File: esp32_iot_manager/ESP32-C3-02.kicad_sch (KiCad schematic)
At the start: 0 parts

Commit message: esp32 page and datasheets
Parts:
- added C10, C13, C14, C8: 0.1u, Capacitor_THT:C_Disc_D3.0mm_W2.0mm_P2.50mm, symbol PCM_SL_Devices:Capacitor_NP
- added C11: 1u, Capacitor_THT:C_Disc_D3.0mm_W2.0mm_P2.50mm, symbol PCM_SL_Devices:Capacitor_NP
- added C13, C7: 10u, symbol Device:C_Polarized
- added C9: 4.7u, symbol Device:C_Polarized
- added J3: GSD090012SEU, GSD090012SEU:AMPHENOL_GSD090012SEU, symbol GSD090012SEU:GSD090012SEU
- added LED5: LTST-C170GKT, LEDC2012X120N, symbol LTST-C170GKT:LTST-C170GKT
- added LED6: LTST-C170KRKT, LEDC2012X120N, symbol LTST-C170KRKT:LTST-C170KRKT
- added R11: 1K, Resistor_THT:R_Axial_DIN0207_L6.3mm_D2.5mm_P10.16mm_Horizontal, symbol PCM_SL_Resistors:Resistor
- added R12: 22.1K, symbol Device:R
- added R13: 47.5K, symbol Device:R
- added R15, R16, R20, R22: 50, Resistor_THT:R_Axial_DIN0207_L6.3mm_D2.5mm_P10.16mm_Horizontal, symbol PCM_SL_Resistors:Resistor
- added R15, R18: 470, symbol Device:R
- added R19: 10K, Resistor_THT:R_Axial_DIN0207_L6.3mm_D2.5mm_P10.16mm_Horizontal, symbol PCM_SL_Resistors:Resistor
- added U3: ESP32-C3-WROOM-02-H4, ESP32-C3-WROOM-02-H4:MODULE_ESP32-C3-WROOM-02-H4, symbol ESP32-C3-WROOM-02-H4:ESP32-C3-WROOM-02-H4
- added U4: CP2102N-Axx-xQFN20, Package_DFN_QFN:SiliconLabs_QFN-20-1EP_3x3mm_P0.5mm, symbol Interface_USB:CP2102N-Axx-xQFN20
- added U5: USBLC6-2P6, PCM_Package_TO_SOT_SMD_AKL:SOT-666, symbol PCM_Diode_TVS_AKL:USBLC6-2P6
- added U6: W25Q32JVSSIQ, W25Q32JVSSIQ:SOIC127P790X216-8N, symbol W25Q32JVSSIQ:W25Q32JVSSIQ
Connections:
- new net: R11.1, U4.9 (~{RST})
- new net: C11.2, R12.2, R13.1, U4.8 (VBUS)
- new net: R20.2, U3.5 (IO6)
- new net: LED6.1 (K), R18.1
- new net: LED5.1 (K), R15.2
- new net: R18.2, U4.19 (~{RXT}/GPIO.3)
- new net: R15.1, U4.20 (~{TXT}/GPIO.2)
- new net: R15.1, U3.6 (IO7)
- new net: J3.7 (DAT0), R16.2
- new net: C14.2, U6.8 (VCC)
- new net: R22.1, U6.2 (DO(IO1))
- new net 3.3V: C10.1, C13.1, C13.2, C7.1, C8.2, C9.1, J3.4 (VDD1), LED5.2 (A), LED6.2 (A), R11.2, R19.1, U3.1 (3V3), U4.6 (VDD), U4.7 (VREGIN), U6.3 (~{WP}(IO2)), U6.7 (~{HOLD}/~{RESET}(IO3))
- new net BOOT: U3.8 (IO9)
- new net CS: U3.10 (IO10), U6.1 (~{CS})
- new net CS_SD: J3.1 (CD/DAT3), R19.2, U3.18 (IO0)
- new net DTS: U4.15 (~{CTS})
- new net EN: U3.2 (EN)
- new net GND: C10.2, C11.1, C13.1, C13.2, C14.1, C7.2, C8.1, C9.2, J3.3 (VSS1), J3.6 (VSS2), J3.8 (DAT1), J3.9 (DAT2), J3.G1 (SHIELD_GND), J3.G2 (SHIELD_GND), J3.G3 (SHIELD_GND), J3.G4 (SHIELD_GND), R13.2, U3.19 (GND), U3.20 (GND), U3.21 (GND), U3.22 (GND), U3.23 (GND), U3.24 (GND), U3.25 (GND), U3.26 (GND), U3.27 (GND), U3.28 (GND), U3.29 (GND), U3.30 (GND), U3.31 (GND), U3.32 (GND), U3.33 (GND), U3.34 (GND), U3.35 (GND), U3.36 (GND), U3.37 (GND), U3.38 (GND), U3.39 (GND), U3.9 (GND), U4.12 (GND), U4.21 (GND), U4.3 (GND), U5.2 (VN), U6.4 (GND)
- new net GPI019: U3.14 (IO19)
- new net GPIO18: U3.13 (IO18)
- new net GPIO8: U3.7 (IO8)
- new net MIC_OUT: U3.4 (IO5)
- new net MISO_DO: R16.1, R22.2, U3.16 (IO2)
- new net MOSI_DI: J3.2 (CMD), R15.2, U6.5 (DI(IO0))
- new net PHOTO_C: U3.17 (IO1)
- new net RTS: U4.16 (~{RTS})
- new net RX_TX: U3.11 (RXD), U4.17 (RXD)
- new net SCL: U3.15 (IO3)
- new net SCLK: J3.5 (CLK), R20.1, U6.6 (CLK)
- new net SDA: U3.3 (IO4)
- new net TX_RX: U3.12 (TXD), U4.18 (TXD)
- new net USB_DATA+: U4.4 (D+), U5.3 (L2)
- new net USB_DATA-: U4.5 (D-), U5.1 (L1)
- new net USB_DN: U5.6 (L1)
- new net USB_DP: U5.4 (L2)
- new net V_BUS: R12.1, U5.5 (VP)
- no-connect marks 0 -> 7
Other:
- note added: "ESP32"
- note added: "Flash Memory"
- note added: "SD Card"
- note added: "USB Module"

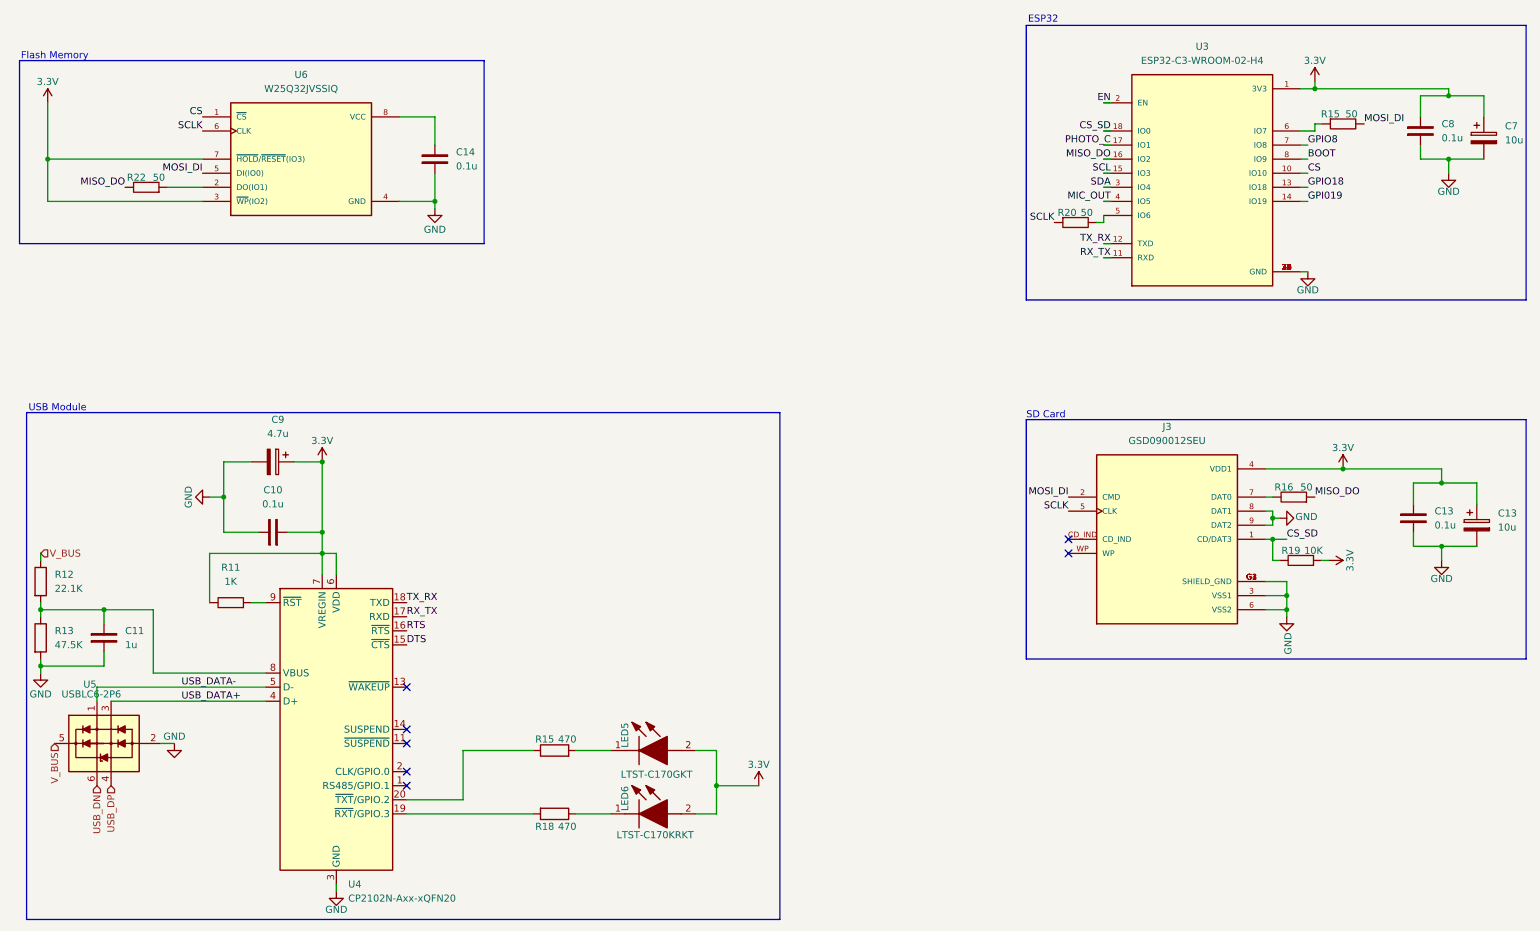
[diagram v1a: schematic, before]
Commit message: finished esp32 sheet, next sensors
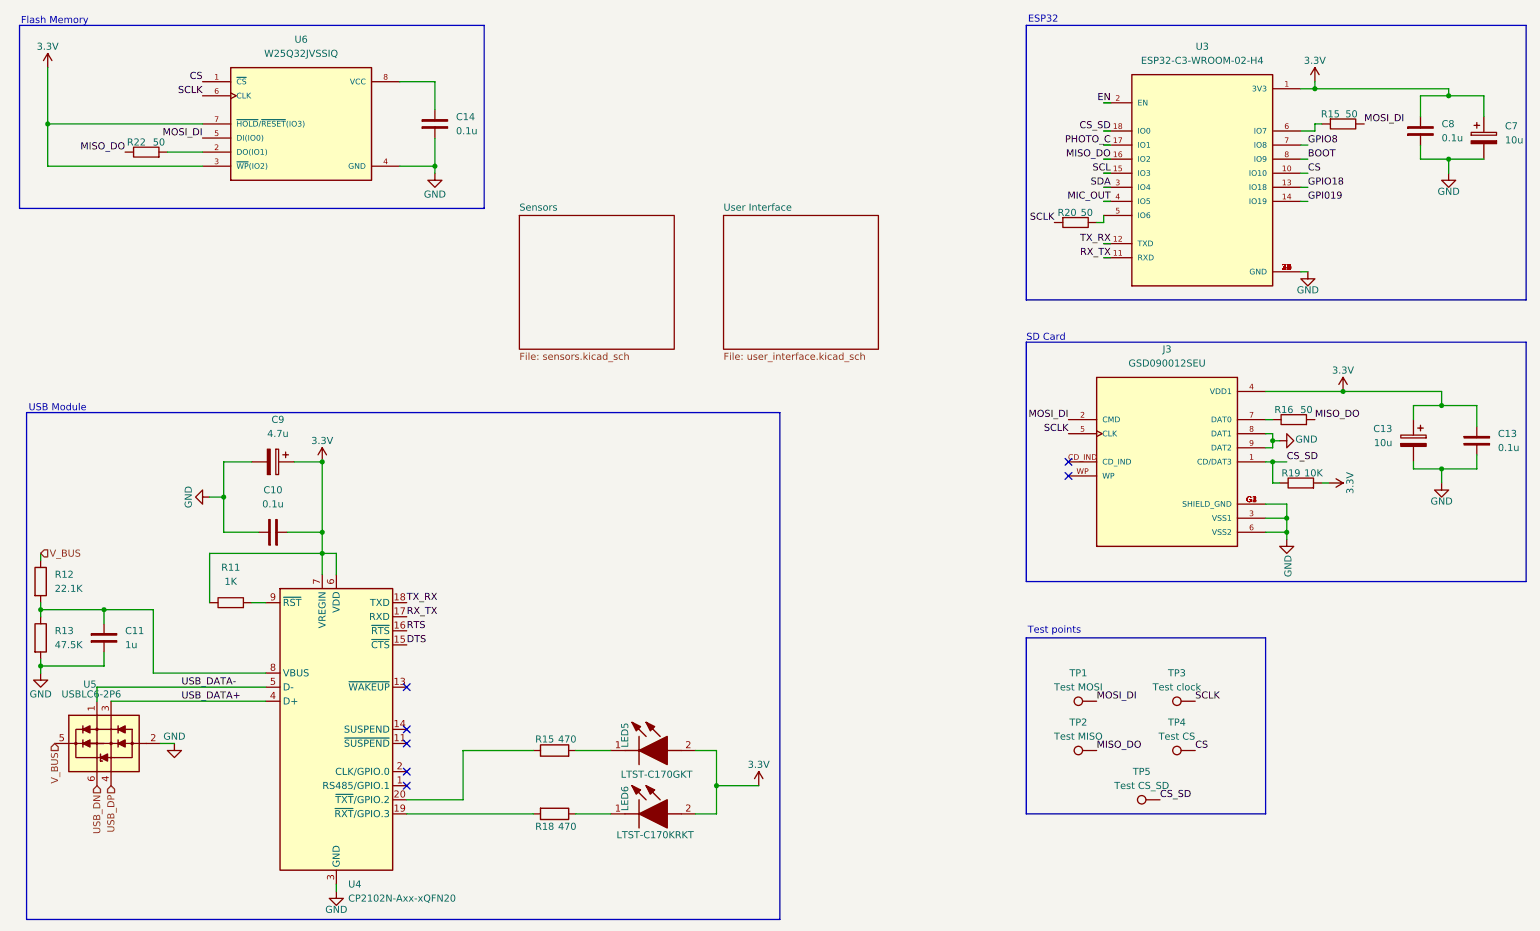
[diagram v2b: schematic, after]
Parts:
- added TP1: Test MOSI, symbol Connector:TestPoint
- added TP2: Test MISO, symbol Connector:TestPoint
- added TP3: Test clock, symbol Connector:TestPoint
- added TP4: Test CS, symbol Connector:TestPoint
- added TP5: Test CS_SD, symbol Connector:TestPoint
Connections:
- net 3.3V: now also C13.1; no longer C13.2
- net CS: now also TP4.1
- net CS_SD: now also TP5.1
- net GND: now also C13.2; no longer C13.1
- net MISO_DO: now also TP2.1
- net MOSI_DI: now also TP1.1
- net SCLK: now also TP3.1
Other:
- added sheet Sensors (sensors.kicad_sch)
- added sheet User Interface (user_interface.kicad_sch)
- note added: "Test points"
- title: (none) -> ESP32 C3 USB and Flash memory SD card
- moved on the sheet: C13, C14, J3, R16, R19, R22, U6
